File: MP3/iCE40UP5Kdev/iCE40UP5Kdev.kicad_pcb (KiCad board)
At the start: 2 copper layers, 29.6 x 52.2 mm, 51 parts, among them J1 USB4105-GF-A, J2 Left, J3 Right, U1 W25Q32JV, U2 MIC5365-1-2YD5, U3 MIC5318-3-3YD5, U4 ICE40UP5K-SG48ITR, X1 IQXO-791

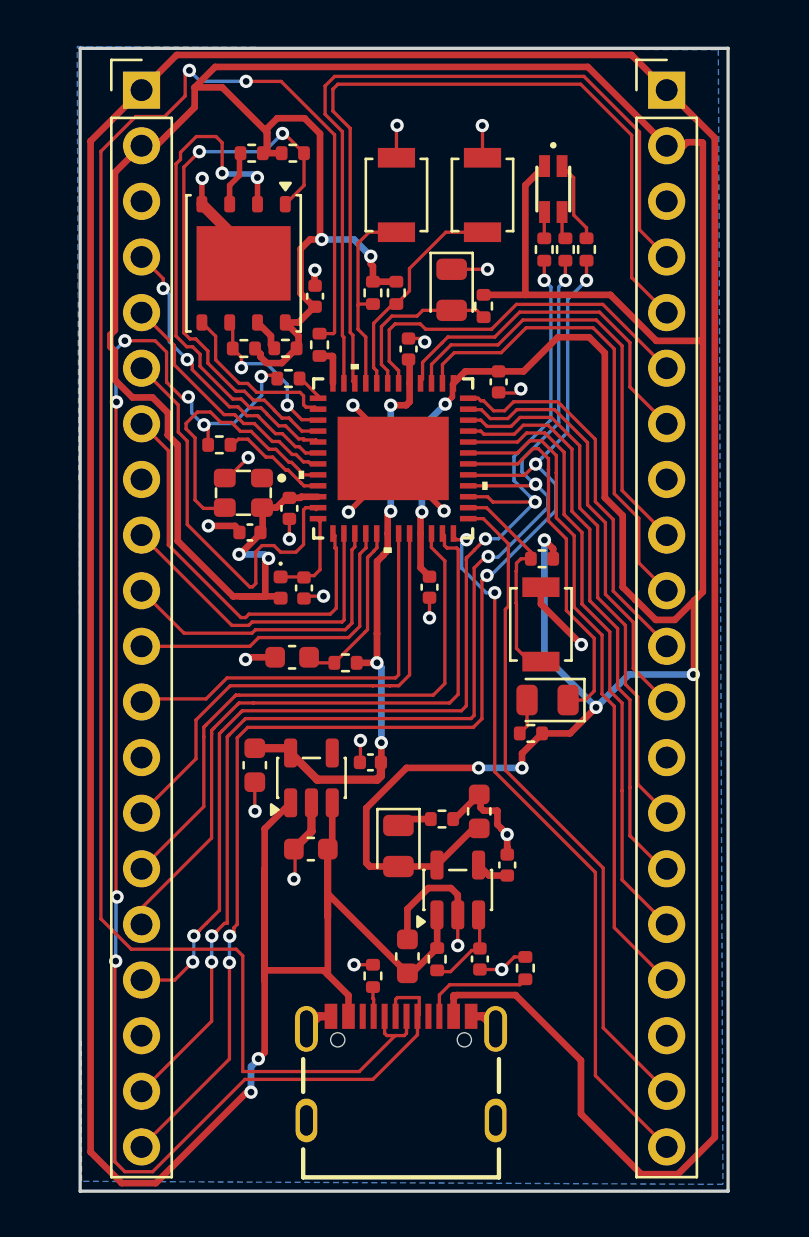
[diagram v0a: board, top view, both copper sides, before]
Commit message: Final Design with PinHeader Labels + Graphics
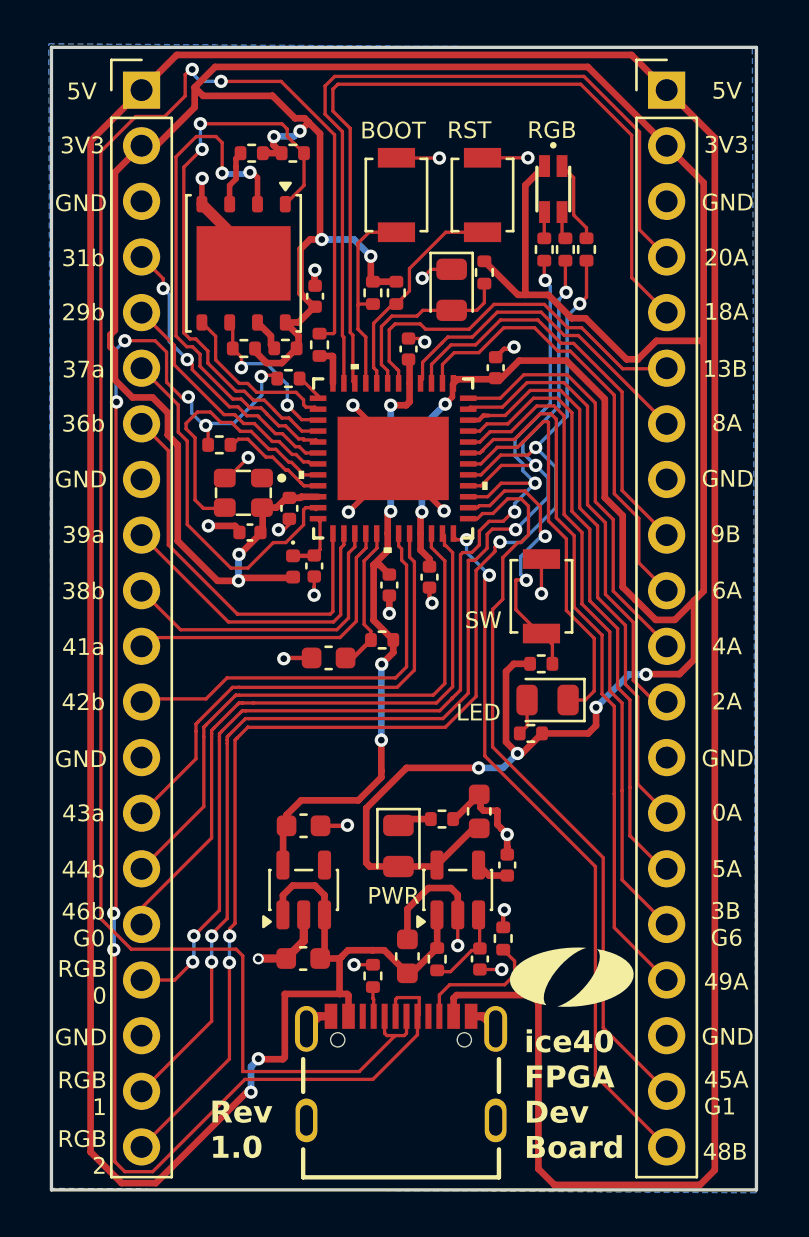
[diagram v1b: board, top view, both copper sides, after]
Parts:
- added G***: LOGO, LOGO, B.Cu at (154.9, 95.2)
- added OlinLogo: G***, Eclectronics:OlinLogo, F.Cu at (165.7, 101.7)
- moved C14 8.14 mm to (157.4, 83.8), turned to 90 degrees
- moved U2 5.13 mm to (153.5, 97.7)
- moved C1 5.01 mm to (153.4, 100.9)
- moved R20 4.80 mm to (164.3, 87.4), turned to 180 degrees
- moved C2 3.55 mm to (153.4, 94.8), turned to 0 degrees
- moved R18 1.97 mm to (157.0, 86.3)
- moved R2 1.69 mm to (162.6, 99.9)
- moved C15 1.67 mm to (154.6, 87.1)
- moved R19 1.53 mm to (161.7, 69.5)
- moved S3 1.28 mm to (164.3, 84.3)
- moved D4 1.12 mm to (153.0, 83.0)
- moved C11 1.11 mm to (153.9, 82.9)
- moved C9 0.66 mm to (162.2, 73.9), turned to -90 degrees
- moved C10 0.46 mm to (159.2, 83.4)
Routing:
- net +5V: track 195.8 -> 181.3 mm
- net +3V3: track 204.9 -> 195.7 mm, vias 11 -> 12
- net /IOT_45a_G1: track 30.4 -> 34.0 mm
- net /IOT_50b: track 10.0 -> 13.3 mm, vias 0 -> 2
- net /IOT_37a: track 18.8 -> 16.5 mm
- net /IOT_49a: track 30.6 -> 32.6 mm
- net /IOT_51a: track 17.0 -> 19.0 mm
- net /IOB_3b_G6: track 29.2 -> 31.2 mm
- net /IOB_2a: track 19.8 -> 21.7 mm
- net /IOB_5a: track 26.5 -> 28.4 mm
- net GND: track 56.0 -> 54.2 mm, vias 24 -> 25
- net /IOB_0a: track 24.3 -> 26.1 mm
- net +1V2: track 27.7 -> 29.5 mm
- net Net-(D4-K): track 4.32 -> 2.80 mm
- net /IOB_4a: track 17.6 -> 19.1 mm
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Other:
- board size 29.6 x 52.2 mm -> 32.2 x 52.2 mm
- board text added: "0A"
- board text added: "13B"
- board text added: "18A"
- board text added: "20A"
- board text added: "29b"
- board text added: "2A"
- board text added: "31b"
- board text added: "36b"
- board text added: "37a"
- board text added: "38b"
- board text added: "39a"
- board text added: "3B G6"
- board text added: "3V3"
- board text added: "41a"
- board text added: "42b"
- board text added: "43a"
- board text added: "44b"
- board text added: "45A G1"
- board text added: "46b G0"
- board text added: "48B"
- board text added: "49A"
- board text added: "4A"
- board text added: "5A"
- board text added: "5V"
- board text added: "6A"
- board text added: "8A"
- board text added: "9B"
- board text added: "BOOT"
- board text added: "By"
- board text added: "Designed Jun Park"
- board text added: "GND"
- board text added: "LED"
- board text added: "PWR"
- board text added: "RGB"
- board text added: "RGB 0"
- board text added: "RGB 1"
- board text added: "RGB 2"
- board text added: "RST"
- board text added: "Rev 1.0"
- board text added: "SW"
- board text added: "ice40 FPGA Dev Board"
